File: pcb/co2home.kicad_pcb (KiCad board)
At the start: 2 copper layers, 40 x 70 mm, 20 parts, among them J1 eflashy32, J2 MH-Z19 L, J3 USBC, J4 MH-Z19 R, J5 JST-PH, SW1 RESET, U1 ESP32-C3-MINI-1, U4 AMS1117-3.3

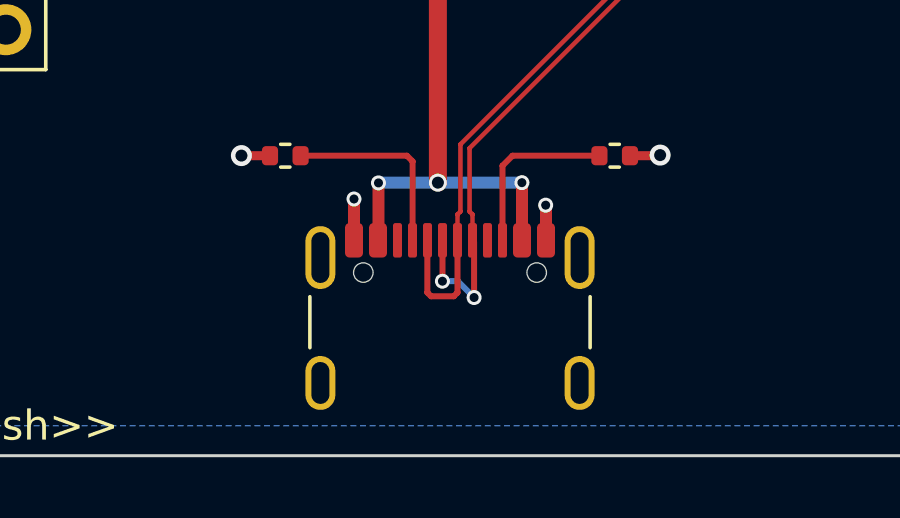
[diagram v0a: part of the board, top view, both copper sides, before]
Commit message: PN for headers
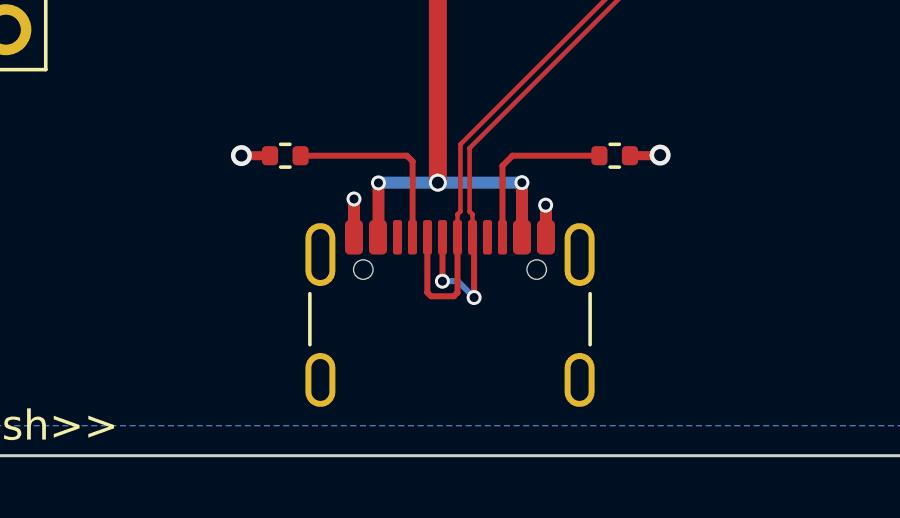
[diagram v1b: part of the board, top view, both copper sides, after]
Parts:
- moved J3 0.10 mm to (134.9, 101.1)
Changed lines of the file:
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@@
     (descr "Through hole straight socket strip, 1x05, 2.54mm pitch, single row (from Kicad 4.0.7), script generated")
     (tags "Through hole socket strip THT 1x05 2.54mm single row")
+    (property "LCSC" "C50950")
     (property "Sheetfile" "co2home.kicad_sch")
     (property "Sheetname" "")
@@
   )
   (footprint "Connector_USB:USB_C_Receptacle_GCT_USB4105-xx-A_16P_TopMnt_Horizontal" (layer "F.Cu")
-    (at 134.925 101.2)
+    (at 134.925 101.1)
     (descr "USB 2.0 Type C Receptacle, GCT, 16P, top mounted, horizontal, 5A: https://gct.co/files/drawings/usb4105.pdf")
     (tags "USB C Type-C Receptacle SMD USB 2.0 16P 16C USB4105-15-A USB4105-15-A-060 USB4105-15-A-120 USB4105-GF-A USB4105-GF-A-060 USB4105-GF-A-120")
@@
     (descr "Through hole straight socket strip, 1x04, 2.54mm pitch, single row (from Kicad 4.0.7), script generated")
     (tags "Through hole socket strip THT 1x04 2.54mm single row")
-    (property "Sheetfile" "co2home.kicad_sch")
-    (property "Sheetname" "")
+    (property "LCSC" "C2718488")
+    (property "Sheetfile" "co2home.kicad_sch")
+    (property "Sheetname" "")
